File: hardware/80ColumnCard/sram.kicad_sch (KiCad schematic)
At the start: 7 parts, among them U10 6116, U10N28 '32 - '256, U10N32 '512, U10W24 6116, U10W28 '32 - '256, U10W32 '512, X21 A11/WE

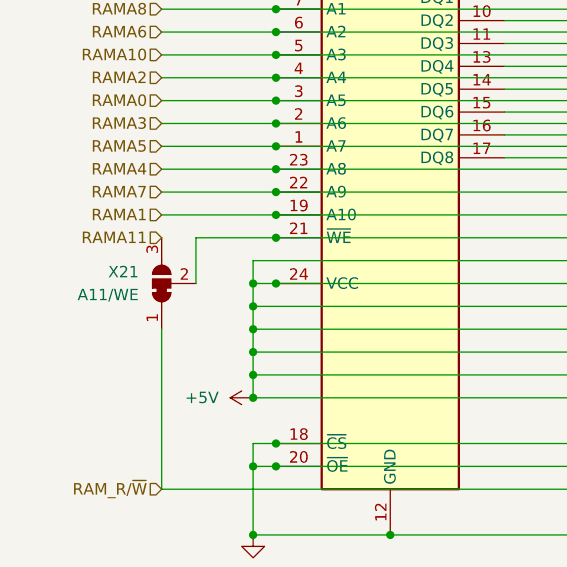
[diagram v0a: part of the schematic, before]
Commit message: Kicad 7, miscellaneous tweaks
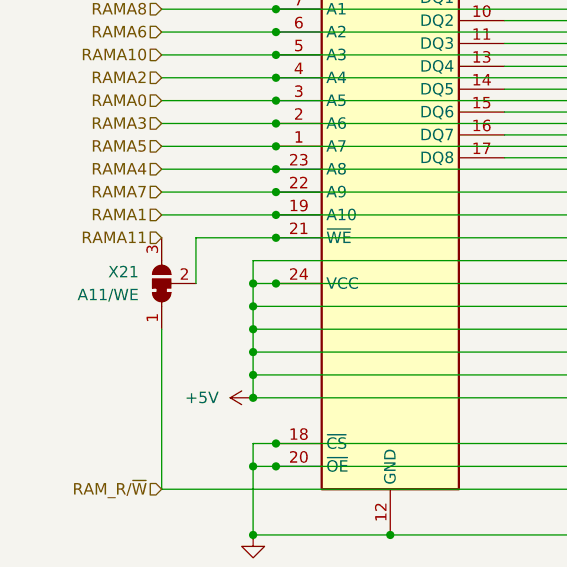
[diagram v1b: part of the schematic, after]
